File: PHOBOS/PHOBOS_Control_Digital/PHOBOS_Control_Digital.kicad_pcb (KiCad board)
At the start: 4 copper layers, 35.6 x 58.4 mm, 71 parts, among them J12 PWR, J14 PS1-2, J15 PS3-4, J2 RF_OUT, J3 USB4056-03-A_REVA2, J4 Screw_Terminal_01x02, J8 BOOT, U1 SX1280IMLTRT, U2 W25Q128JVSIQ, U3 NCP1117-3.3_SOT223, U4 RP2040, U5 TPS60403DBV, Y1 C1E-52.000-10-1012-X-M, Y2 ABM8-272-T3

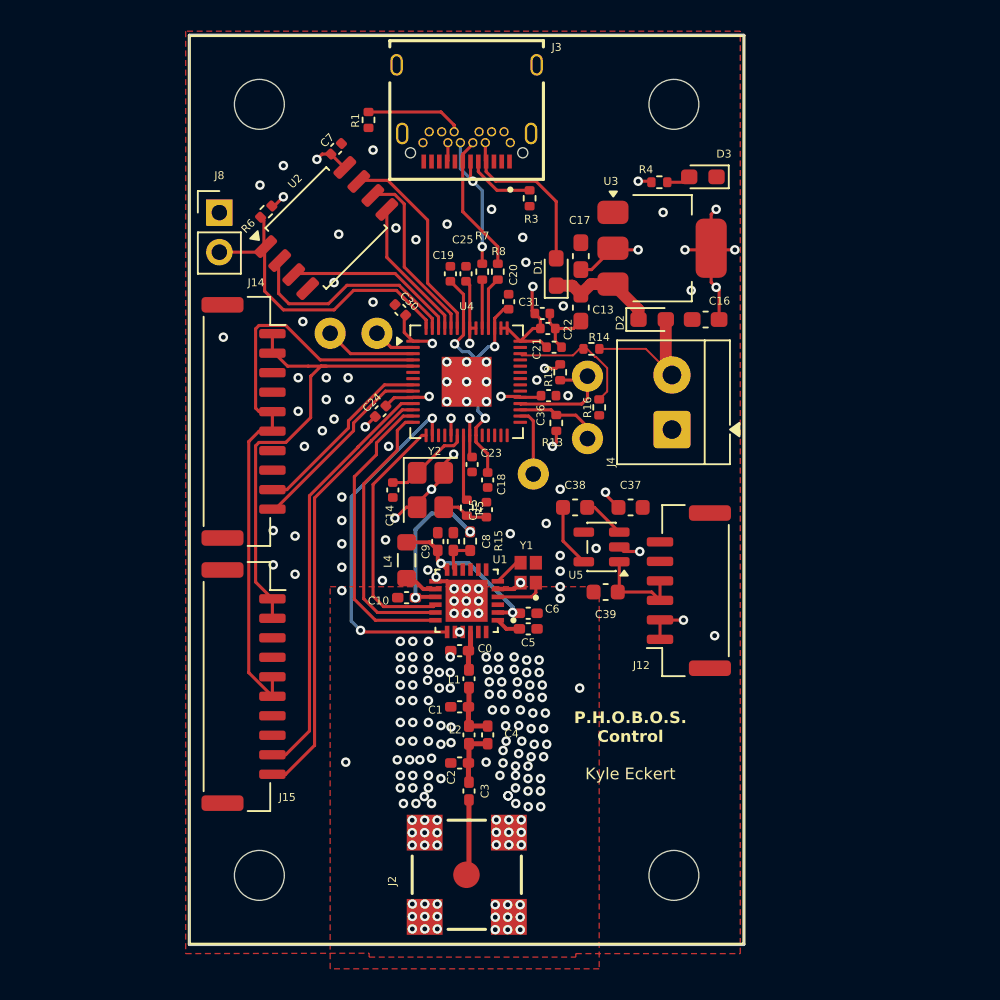
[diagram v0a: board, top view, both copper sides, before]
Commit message: review submission files created
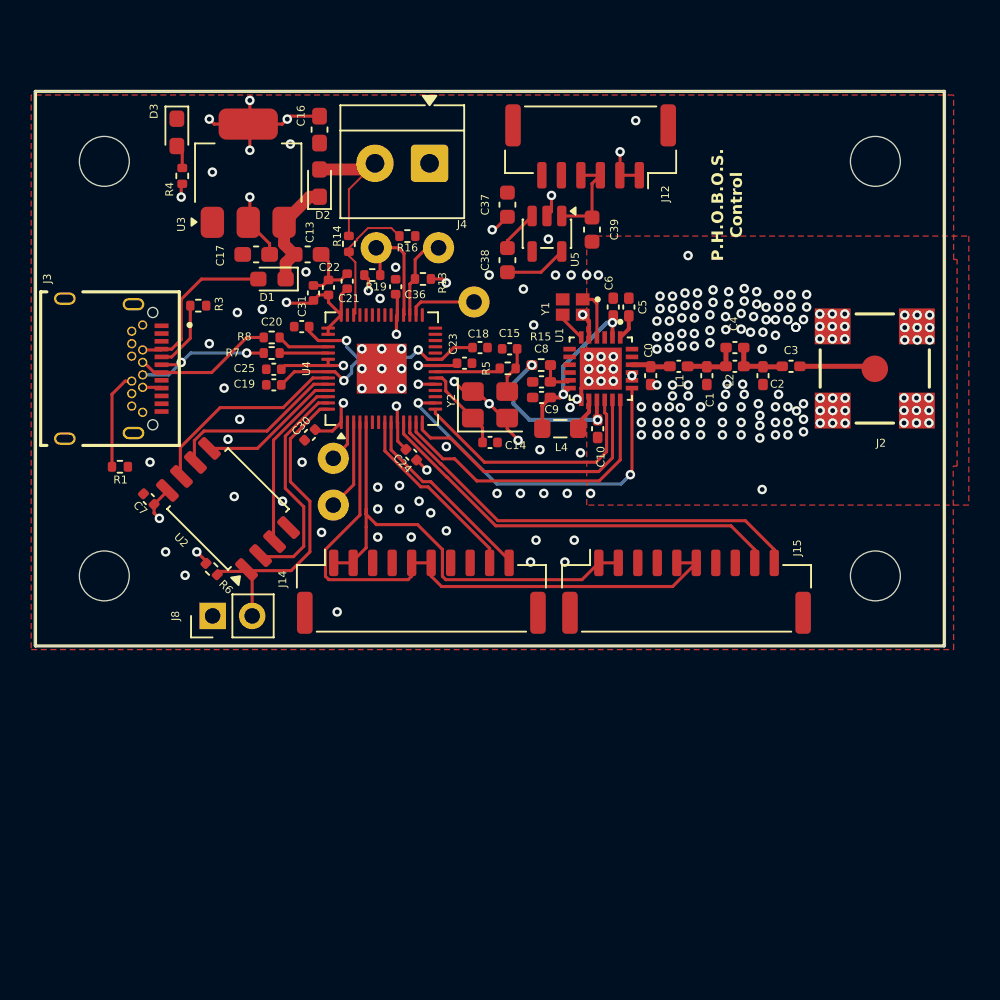
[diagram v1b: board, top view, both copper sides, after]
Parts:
- J4: value Screw_Terminal_01x02 -> BATT
- moved H4 47.6 mm to (184.3, 85.1), turned to 90 degrees
- moved H2 43.9 mm to (184.3, 111.7), turned to 90 degrees
- moved J2 41.7 mm to (184.3, 98.4), turned to 180 degrees
- moved H1 36.7 mm to (134.9, 85.1), turned to 90 degrees
- moved C3 34.2 mm to (178.9, 98.2), turned to 0 degrees
- moved D3 33.8 mm to (139.5, 83.2), turned to -90 degrees
- moved J3 32.3 mm to (132.3, 98.4), turned to -90 degrees
- moved H3 31.8 mm to (134.9, 111.7), turned to 90 degrees
- moved C2 31.5 mm to (177.1, 98.8), turned to -90 degrees
- moved R4 30.6 mm to (139.9, 86.0), turned to -90 degrees
- moved C4 29.5 mm to (175.3, 97.0), turned to 0 degrees
- moved J12 29.2 mm to (166.0, 84.1), turned to 180 degrees
- moved L2 29.1 mm to (175.3, 98.2), turned to 0 degrees
- moved J15 29.0 mm to (172.2, 112.7), turned to 0 degrees
- moved C16 27.6 mm to (148.7, 83.1), turned to -90 degrees
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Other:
- board size 35.6 x 58.4 mm -> 58.4 x 35.6 mm
- board text removed: "Kyle Eckert"
